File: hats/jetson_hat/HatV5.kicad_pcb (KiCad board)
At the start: 4 copper layers, 62 x 31.5 mm, 31 parts, among them J1 CLIK-Mate 502584, J2 CLIK-Mate 502584, J3 CLIK-Mate 502584, J4 CLIK-Mate 502584, J5 02x20 2.54 mm Female Socket, J6 24 Pin Header, U1 TCAN1051HGVDRBRQ1, U2 PESD2CANFD27V-TR, U3 TCAN1051HGVDRBRQ1, U4 PESD2CANFD27V-TR

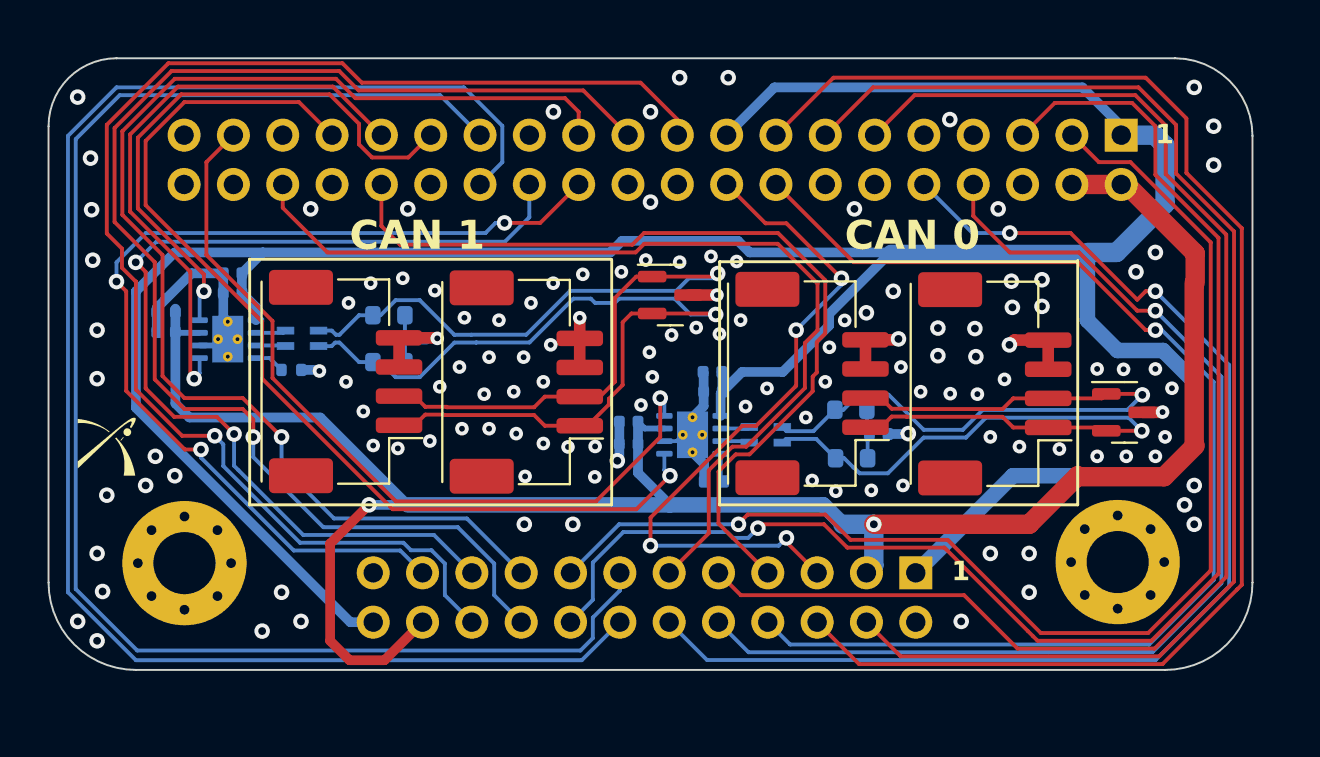
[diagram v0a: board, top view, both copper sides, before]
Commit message: impedance checked and traces spaced out
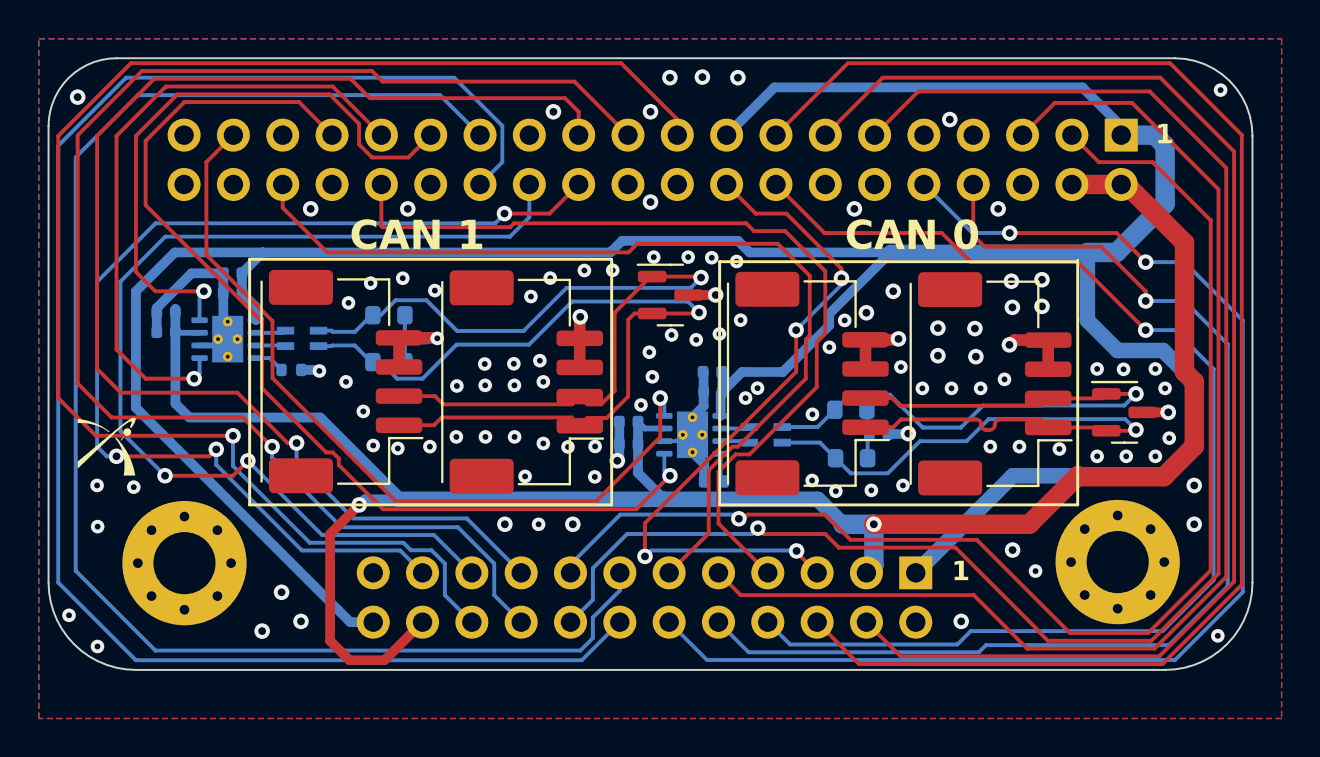
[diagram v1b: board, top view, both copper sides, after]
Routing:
- net /SPI1_MOSI: track 70.8 -> 76.9 mm
- net /SPI1_MISO: track 69.0 -> 73.1 mm
- net /SPI1_CS0: track 51.7 -> 55.6 mm
- net /SPI1_SCK: track 63.5 -> 66.7 mm
- net /UART1_TX: track 56.4 -> 59.1 mm
- net /UART1_RX: track 62.5 -> 65.1 mm
- net /CAN0_DOUT: track 30.1 -> 32.5 mm
- net /SPI1_CS1: track 51.3 -> 53.6 mm
- net /CAN BUS 0/CH0-: track 45.5 -> 43.4 mm
- net /CAN BUS 0/CH0+: track 44.7 -> 42.7 mm
- net /GPIO27_PWM2: track 72.9 -> 74.7 mm
- net /CAN0_DIN: track 29.3 -> 31.0 mm
- net /PWM01: track 65.9 -> 67.3 mm
- net /I2C_GP2_DAT: track 77.9 -> 76.8 mm
- net /I2C_GP5_DAT: track 64.4 -> 65.5 mm
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- added copper zone on B.Cu, net GND
- added copper zone on F.Cu, net GND
